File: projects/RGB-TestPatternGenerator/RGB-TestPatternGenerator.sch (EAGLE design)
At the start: 15 parts, among them IC1 7805TV, IC2 7809TV, IC3 4060N, IC4 4040N, IC5 74HC10N, IC6 4082N, IC7 74HC32N, IC8 74LS157N

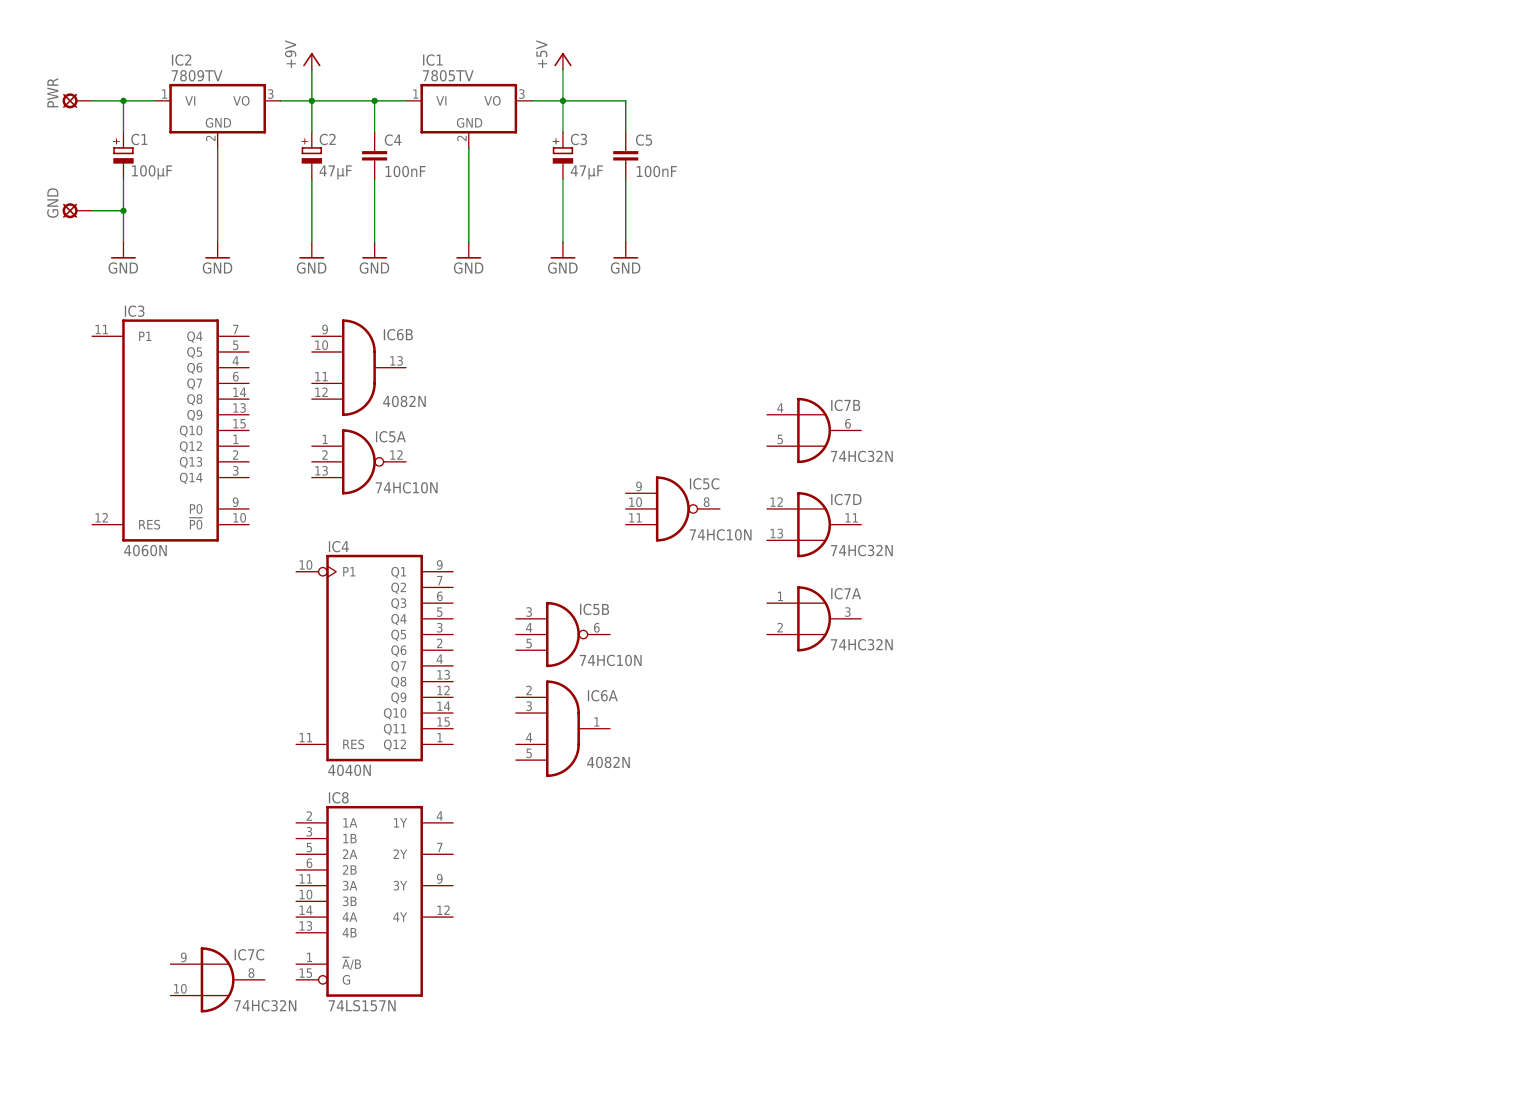
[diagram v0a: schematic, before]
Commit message: feat: rgb schematic
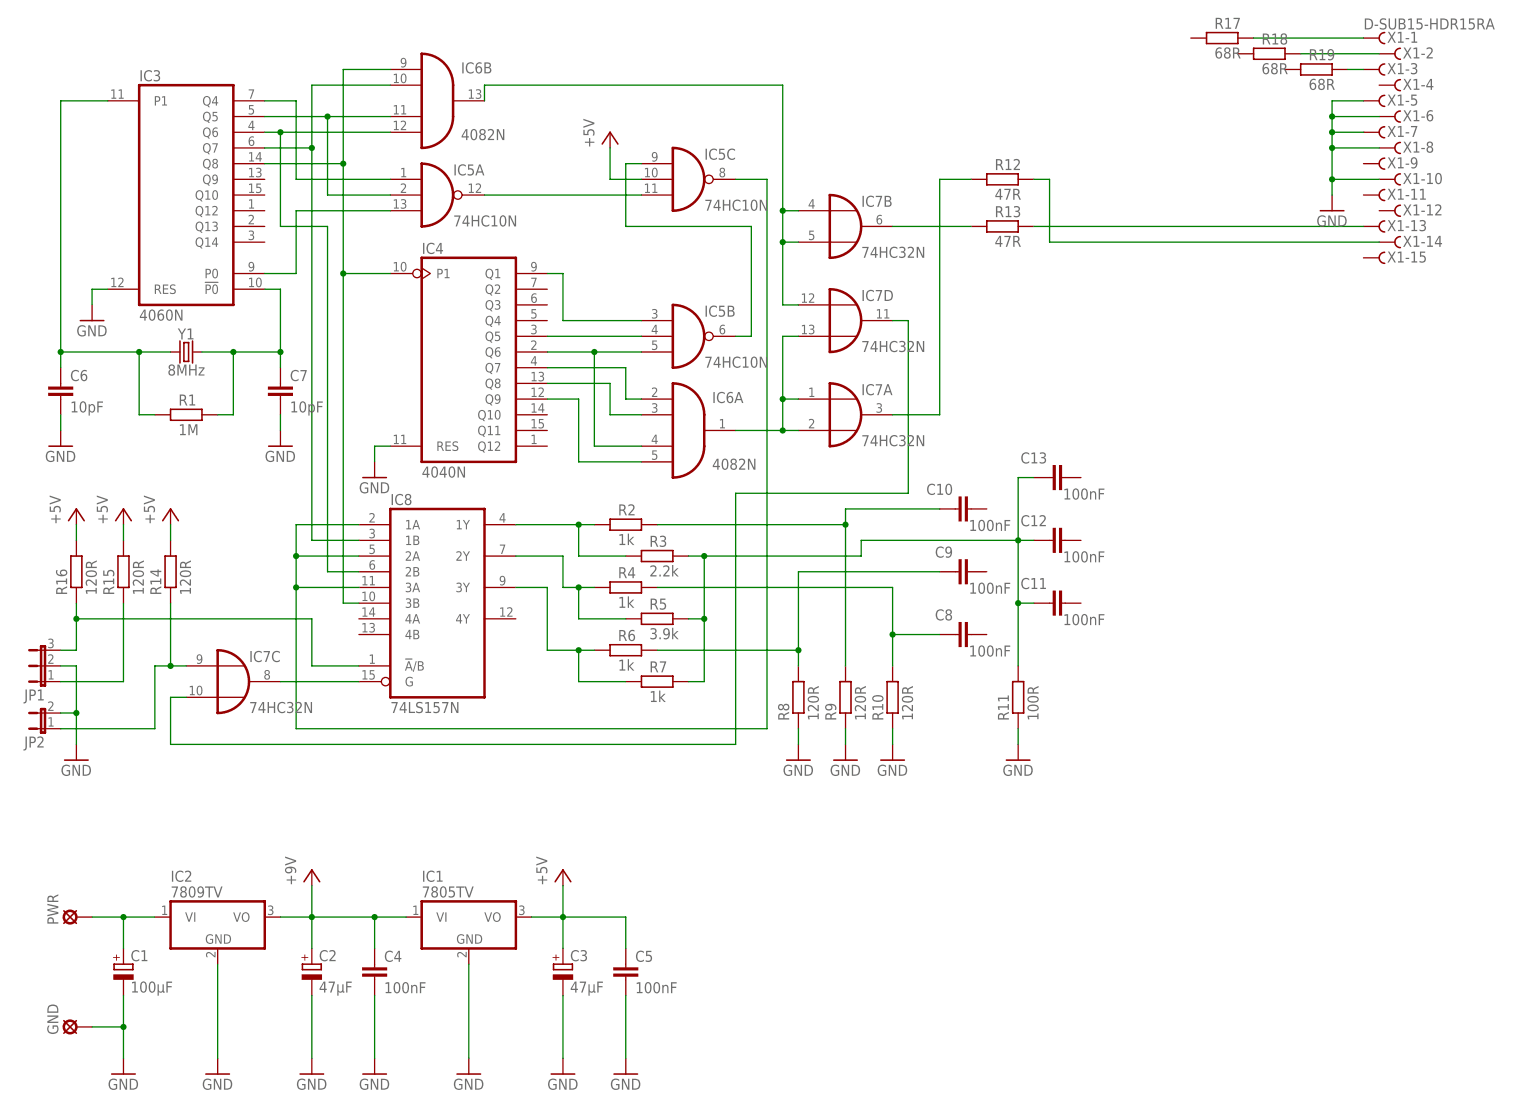
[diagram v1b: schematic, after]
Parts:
- added C10, C11, C12, C13, C8, C9: 100nF, rcl:C-EU050-024X044
- added C6, C7: 10pF, rcl:C-EU050-024X044
- added JP1: (no value), jumper:JP2E
- added JP2: (no value), jumper:JP1E
- added R1: 1M, rcl:R-EU_0207/10
- added R10, R14, R15, R16, R8, R9: 120R, rcl:R-EU_0207/10
- added R11: 100R, rcl:R-EU_0207/10
- added R12, R13: 47R, rcl:R-EU_0207/10
- added R17, R18, R19: 68R, rcl:R-EU_0207/10
- added R2, R4, R6, R7: 1k, rcl:R-EU_0207/10
- added R3: 2.2k, rcl:R-EU_0207/10
- added R5: 3.9k, rcl:R-EU_0207/10
- added X1: D-SUB15-HDR15RA, con-thomas-betts:D-SUB15-HDR15RA
- added Y1: 8MHz, SparkFun-Clocks:CRYSTALPTH-HC49US
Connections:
- new net N$10: IC5C.O, IC8A.1A, IC8A.2A, IC8A.3A
- new net N$11: IC7C.O, IC8A.G
- new net N$12: IC4A.Q6, IC5B.I2, IC6A.I2
- new net N$13: IC4A.Q5, IC5B.I1
- new net N$14: IC4A.Q1, IC5B.I0
- new net N$15: IC4A.Q7, IC6A.I0
- new net N$16: IC4A.Q8, IC6A.I1
- new net N$17: IC5A.O, IC5C.I2
- new net N$18: IC4A.Q9, IC6A.I3
- new net N$19: IC5B.O, IC5C.I0
- new net N$2: C6.1, IC3A.P1, R1.1, Y1.1
- new net N$20: IC6A.O, IC7A.I0, IC7A.I1, IC7D.I1
- new net N$21: IC8A.1Y, R2.1, R3.1
- new net N$22: IC6B.O, IC7B.I0, IC7B.I1, IC7D.I0
- new net N$23: IC8A.2Y, R4.1, R5.1
- new net N$24: IC8A.3Y, R6.1, R7.1
- new net N$25: C11.1, C12.1, C13.1, R11.2, R3.2, R5.2, R7.2
- new net N$26: C9.1, R6.2, R8.2
- new net N$27: C10.1, R2.2, R9.2
- new net N$28: C8.1, R10.2, R4.2
- new net N$29: IC7C.I1, IC7D.O
- new net N$3: C7.1, IC3A.!P0, R1.2, Y1.2
- new net N$30: IC7B.O, R13.1
- new net N$31: IC7A.O, R12.1
- new net N$32: IC7C.I0, JP2.1, R14.1
- new net N$33: IC8A.!A!/B, JP1.3, R16.1
- new net N$34: R13.2, X1-13.F
- new net N$35: R12.2, X1-14.F
- new net N$36: R17.2, X1-1.F
- new net N$37: JP1.1, R15.1
- new net N$38: R18.2, X1-2.F
- new net N$39: R19.2, X1-3.F
- new net N$4: IC3A.Q5, IC5A.I1, IC6B.I2
- new net N$5: IC3A.Q6, IC6B.I3, IC8A.2B
- new net N$6: IC3A.Q4, IC5A.I0
- new net N$7: IC3A.P0, IC5A.I2
- new net N$8: IC3A.Q7, IC6B.I1, IC8A.1B
- new net N$9: IC3A.Q8, IC4A.P1, IC6B.I0, IC8A.3B
- net GND: now also C6.2, C7.2, IC3A.RES, IC4A.RES, JP1.2, JP2.2, R10.1, R11.1, R8.1, R9.1, X1-10.F, X1-5.F, X1-6.F, X1-7.F, X1-8.F
- net VCC: now also IC5C.I1, R14.2, R15.2, R16.2
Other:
- moved on the sheet: C1, C2, C3, C4, C5, GND, IC1, IC2, IC3, IC4, IC5A, IC5B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
